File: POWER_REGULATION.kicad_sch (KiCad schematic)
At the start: 41 parts, among them J1 PJ-102AH, J17 Conn_01x02_Pin, J2 Conn_01x01_Pin, J3 Conn_01x03_Pin, Q7 DMG2305UX-13, U14 TLV62130RGTT, U15 LP5907MFX-3.3, U16 REF3012

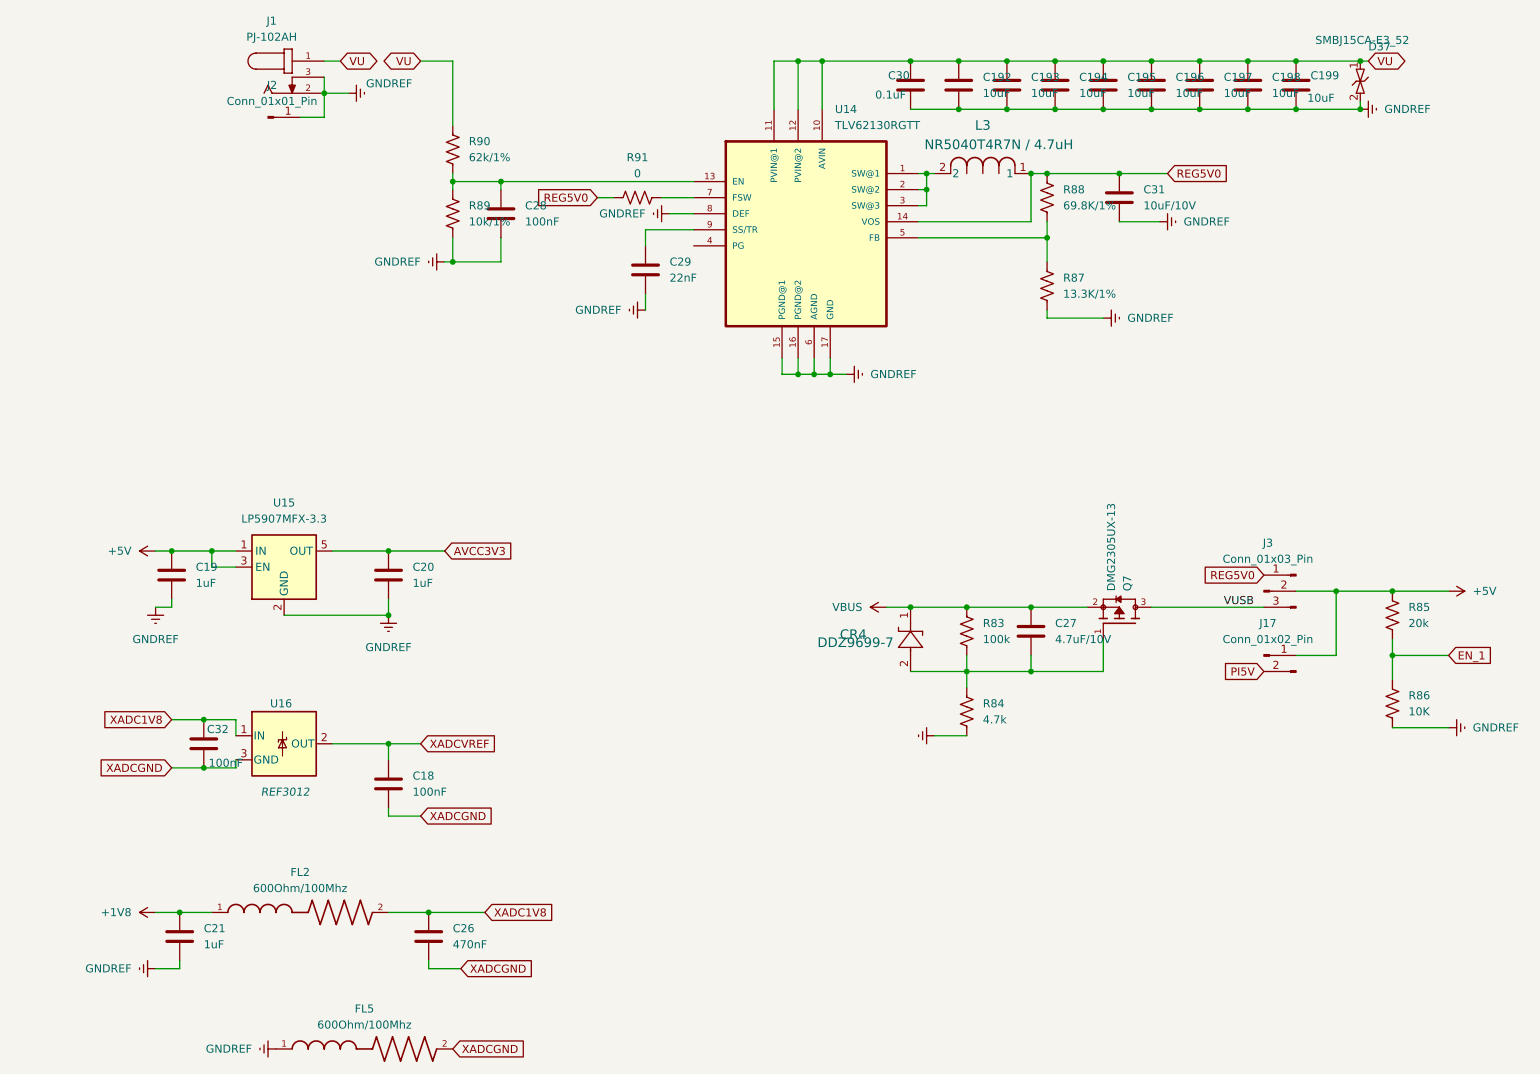
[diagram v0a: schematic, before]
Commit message: new layout by abdul
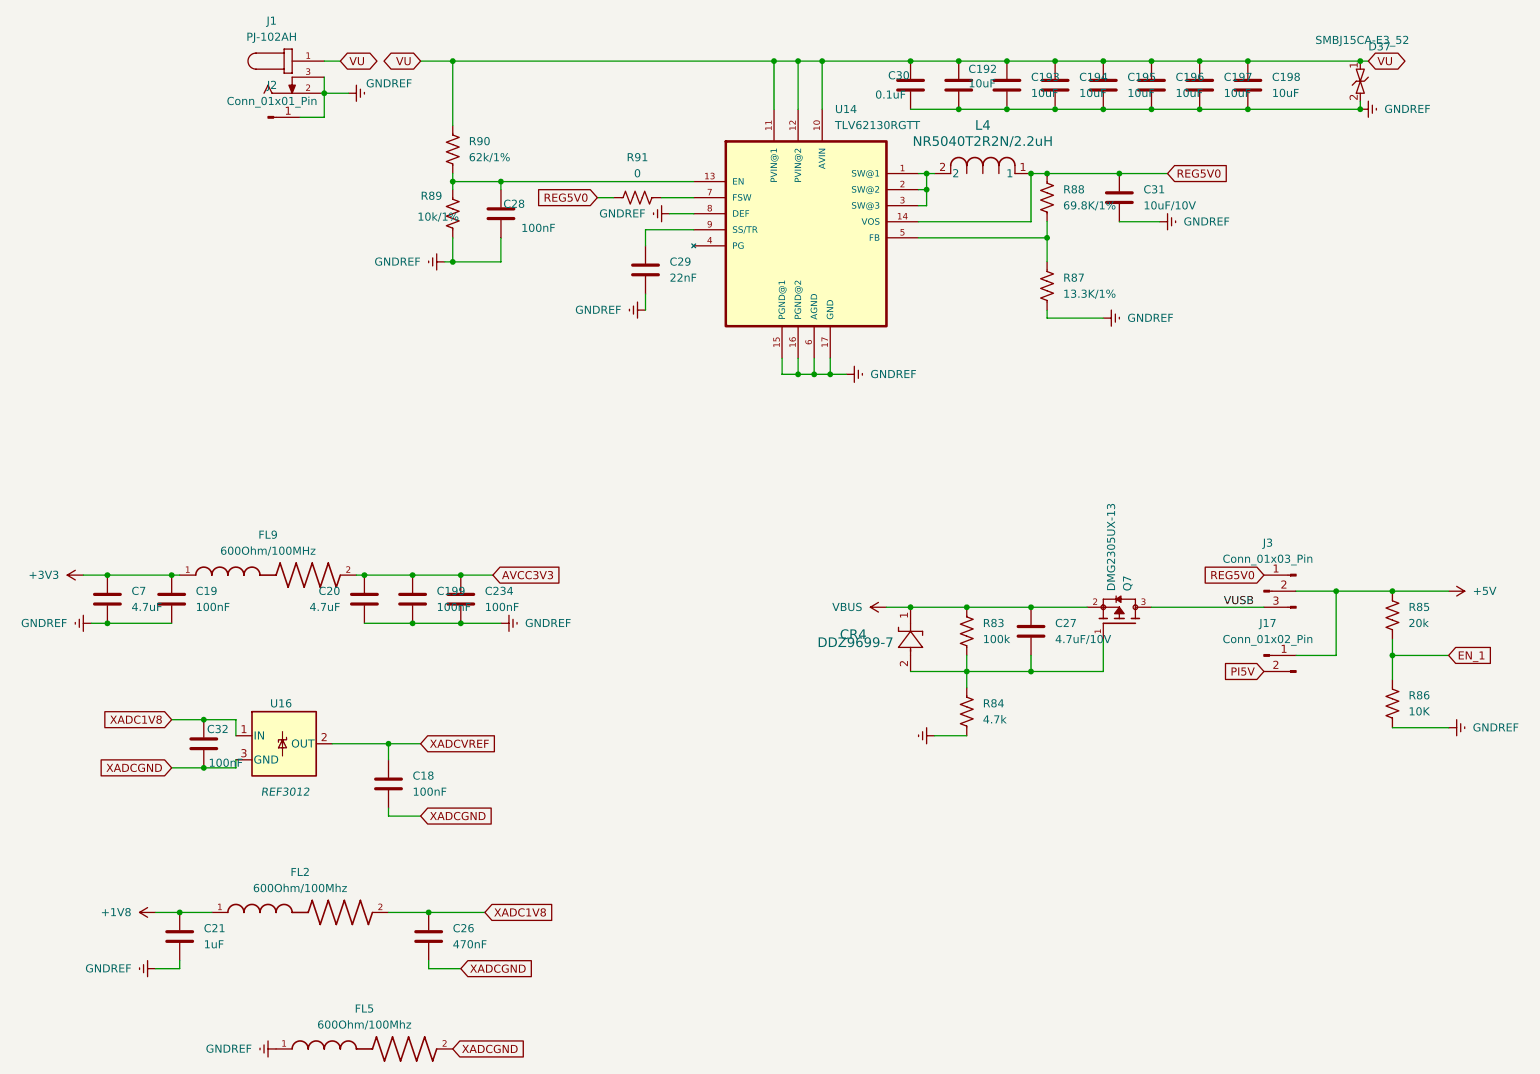
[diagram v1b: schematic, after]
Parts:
- removed L3: NR5040T4R7N / 4.7uH, footprints:IND_TAIYO_NR5040_TAY, symbol NR5040T4R7N:NR5040T4R7N
- removed U15: LP5907MFX-3.3, footprints:SOT-23-5, symbol Regulator_Linear:LP5907MFX-3.3
- added C234: 100nF, footprints:C_0201_0603Metric, symbol Device:C
- added C7: 4.7uF, footprints:C_0402, symbol Device:C
- added FL9: 600Ohm/100MHz, footprints:BEADC1608X95N, symbol BLM18AG601SZ1D:BLM18AG601SZ1D
- added L4: NR5040T2R2N/2.2uH, footprints:IND_TAIYO_NR5040_TAY, symbol 2025-03-04_21-33-04:NR5040T2R2N
- C19: value 1uF -> 100nF; footprint footprints:C_0402 -> footprints:C_0201_0603Metric; LCSC PN c14445 -> c1525
- C192, C193, C194, C195, C196, C197, C198, C29, C31: footprint footprints:C_0402 -> footprints:C_0805
- C199: value 10uF -> 100nF; footprint footprints:C_0402 -> footprints:C_0201_0603Metric; LCSC PN c315248 -> c1525
- C20: value 1uF -> 4.7uF; LCSC PN c14445 -> c23733
- C26: footprint footprints:C_0402 -> footprints:C_0201_0603Metric; LCSC PN c92361 -> C88915
- C28: footprint footprints:C_0402 -> footprints:C_0201_0603Metric
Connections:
- net +5V: no longer C19.1
- net AVCC3V3: now also C199.1, C234.1, FL9.2
- net GNDREF: now also C234.2, C7.2
- net REG5V0: now also L4.1
- net VU: no longer C199.1
- net at U14.1 (SW@1), U14.2 (SW@2), U14.3 (SW@3): now also L4.2
- new net +3V3: C19.1, C7.1, FL9.1

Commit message: update
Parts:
- C18, C32: footprint footprints:C_0402 -> footprints:C_0201_0603Metric
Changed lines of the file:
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@@
 			)
 		)
-		(property "Footprint" "footprints:C_0402"
+		(property "Footprint" "footprints:C_0201_0603Metric"
 			(at 55.5752 129.54 0)
 			(effects
@@
 			)
 		)
-		(property "Footprint" "footprints:C_0402"
+		(property "Footprint" "footprints:C_0201_0603Metric"
 			(at 84.7852 135.89 0)
 			(effects
